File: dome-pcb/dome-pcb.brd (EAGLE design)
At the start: 45 x 73 mm, 16 parts, among them K1 CQ1-12V, K5 CQ1-12V, Q1 500mA/300V, Q2 500mA/300V, U1 ESP8266_ESP-01

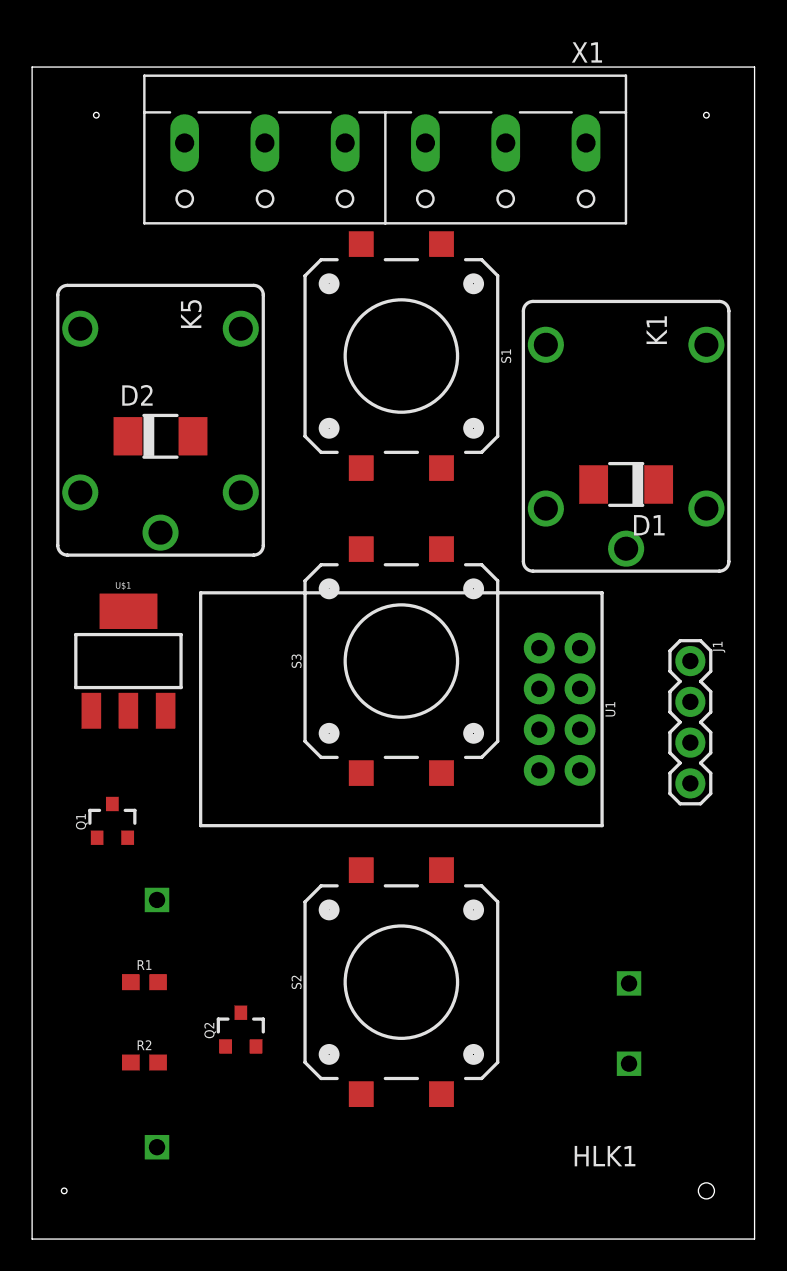
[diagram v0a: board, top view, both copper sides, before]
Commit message: PCB Schematics and board
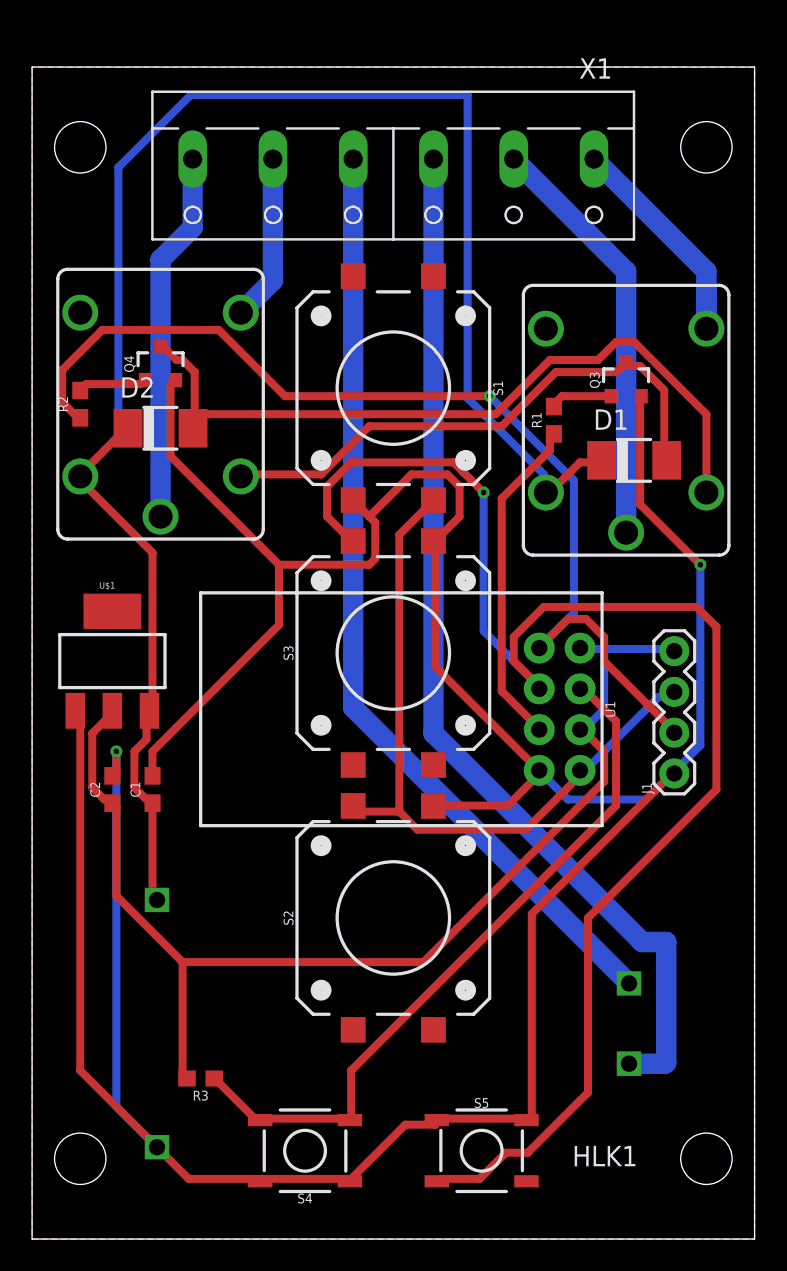
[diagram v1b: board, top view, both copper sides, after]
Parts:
- removed Q1, Q2: 500mA/300V, DiscreteSemi:SOT23-3
- added C1, C2: 10uF, Capacitors:0603
- added Q3, Q4: 600mA/40V, DiscreteSemi:SOT23-3
- added R3: 10k, Resistors:0603
- added S4, S5: (no value), Switches:TACTILE_SWITCH_SMD_5.2MM
- moved R1 43.3 mm to (32.5, 51.0), turned to 90 degrees
- moved R2 41.2 mm to (3.00, 52.0), turned to 90 degrees
- moved J1 7.07 mm to (40.0, 29.0), turned to 90 degrees
- moved S2 4.03 mm to (22.5, 20.0)
- moved S1 2.06 mm to (22.5, 53.0)
- moved D1 1.58 mm to (37.5, 48.5), turned to 0 degrees
- moved X1 1.12 mm to (22.5, 66.0)
- moved K1 1.00 mm to (37.0, 51.0)
- moved K5 1.00 mm to (8.00, 52.0)
- moved U$1 1.00 mm to (5.00, 36.0)
- moved S3 0.71 mm to (22.5, 36.5)
- moved D2 0.50 mm to (8.00, 50.5)
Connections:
- removed net N$1: S1.3
- removed net N$2: S2.3
- removed net N$3: S3.3
- new net 3.3V: C2.1, J1.4, R3.2, U$1.2, U1.2, U1.4
- new net AC1: HLK1.P$1, X1.3
- new net AC2: HLK1.P$2, X1.4
- new net AC_SWITCH_1A: K1.NO, X1.1
- new net AC_SWITCH_1B: K1.C, X1.2
- new net AC_SWITCH_2A: K5.NO, X1.5
- new net AC_SWITCH_2B: K5.C, X1.6
- new net GPIO0: S3.3, S5.3, U1.6
- new net GPIO1: J1.3, S1.3, S2.3, U1.1
- new net GPIO2: R1.1, U1.7
- new net GPIO3: J1.2, R2.1, U1.5
- new net RST: R3.1, S4.3, S4.4, U1.3
- net 5V: now also C1.1, HLK1.P$4, K1.1, U$1.3
- net GND: now also C1.2, C2.2, HLK1.P$3, J1.1, Q3.2, Q4.2, S4.1, S4.2, S5.1, S5.2, U$1.1, U1.8; no longer Q1.2
- net N$10: now also Q4.1
- net N$11: now also Q3.3; no longer Q1.3
- net N$12: now also Q3.1; no longer Q1.1
- net N$9: now also K1.2, Q4.3
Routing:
- net GND: track 0.00 -> 220.7 mm, vias 0 -> 2
- net 5V: track 0.00 -> 108.7 mm
- net GPIO0: track 0.00 -> 90.7 mm, vias 0 -> 1
- net 3.3V: track 0.00 -> 72.6 mm
- net AC1: track 0.00 -> 65.5 mm
- net GPIO3: track 0.00 -> 64.8 mm, vias 0 -> 1
- net AC2: track 0.00 -> 58.5 mm
- net N$9: track 0.00 -> 47.7 mm
- net GPIO1: track 0.00 -> 44.7 mm
- net RST: track 0.00 -> 44.3 mm
- net N$11: track 0.00 -> 34.5 mm
- net AC_SWITCH_1B: track 0.00 -> 26.2 mm
- net AC_SWITCH_2B: track 0.00 -> 23.1 mm
- net GPIO2: track 0.00 -> 20.7 mm
- net AC_SWITCH_1A: track 0.00 -> 16.3 mm
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- added copper zone on layer 1, net GND
- added copper zone on layer 16, net GND
